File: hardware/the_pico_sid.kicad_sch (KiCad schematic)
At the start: 14 parts, among them J1 SWD, U1 4050, U2 SID_6581, U3 4050, U4 4050, U5 Pico

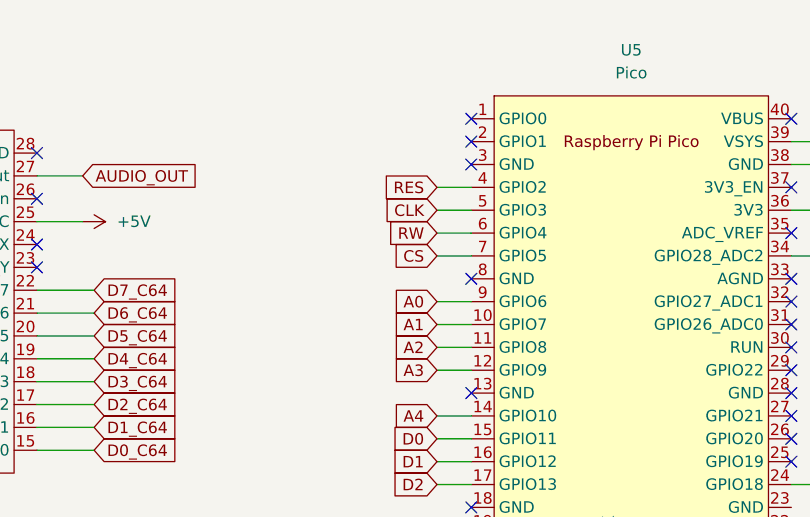
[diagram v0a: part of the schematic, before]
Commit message: Update the_pico_sid.kicad_sch
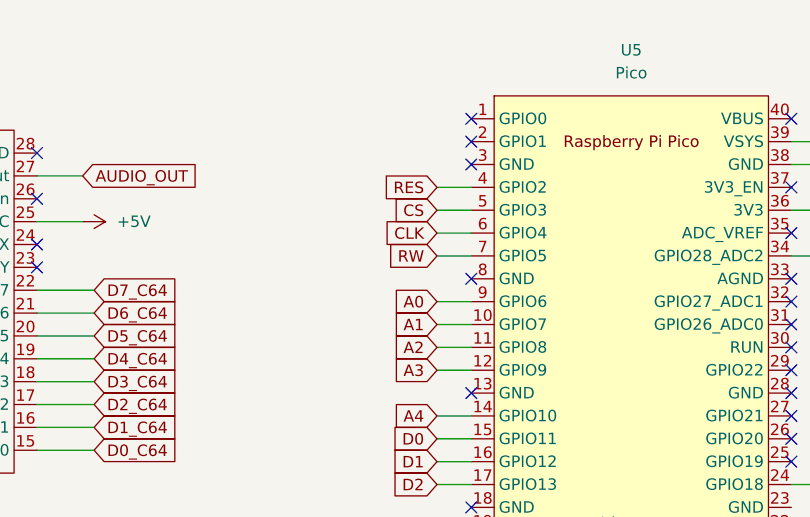
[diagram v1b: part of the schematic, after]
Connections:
- net CLK: now also U5.6 (GPIO4); no longer U5.5 (GPIO3)
- net CS: now also U5.5 (GPIO3); no longer U5.7 (GPIO5)
- net RW: now also U5.7 (GPIO5); no longer U5.6 (GPIO4)
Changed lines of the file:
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@@
     )
   )
-  (global_label "CS" (shape input) (at 104.14 40.64 180) (fields_autoplaced)
-    (effects (font (size 1.27 1.27)) (justify right))
-    (property "Referenzen zwischen Schaltplänen" "${INTERSHEET_REFS}" (id 0) (at 99.2474 40.7194 0)
+  (global_label "CS" (shape input) (at 104.14 35.56 180) (fields_autoplaced)
+    (effects (font (size 1.27 1.27)) (justify right))
+    (property "Referenzen zwischen Schaltplänen" "${INTERSHEET_REFS}" (id 0) (at 99.2474 35.6394 0)
       (effects (font (size 1.27 1.27)) (justify right) hide)
     )
@@
     )
   )
-  (global_label "RW" (shape input) (at 104.14 38.1 180) (fields_autoplaced)
-    (effects (font (size 1.27 1.27)) (justify right))
-    (property "Referenzen zwischen Schaltplänen" "${INTERSHEET_REFS}" (id 0) (at 99.0055 38.1794 0)
+  (global_label "RW" (shape input) (at 104.14 40.64 180) (fields_autoplaced)
+    (effects (font (size 1.27 1.27)) (justify right))
+    (property "Referenzen zwischen Schaltplänen" "${INTERSHEET_REFS}" (id 0) (at 99.0055 40.7194 0)
       (effects (font (size 1.27 1.27)) (justify right) hide)
     )
@@
     )
   )
-  (global_label "CLK" (shape input) (at 104.14 35.56 180) (fields_autoplaced)
-    (effects (font (size 1.27 1.27)) (justify right))
-    (property "Referenzen zwischen Schaltplänen" "${INTERSHEET_REFS}" (id 0) (at 98.1588 35.6394 0)
-      (effects (font (size 1.27 1.27)) (justify right) hide)
-    )
+  (global_label "CLK" (shape input) (at 104.14 38.1 180) (fields_autoplaced)
+    (effects (font (size 1.27 1.27)) (justify right))
+    (property "Referenzen zwischen Schaltplänen" "${INTERSHEET_REFS}" (id 0) (at 98.1588 38.1794 0)
+      (effects (font (size 1.27 1.27)) (justify right) hide)
+    )
